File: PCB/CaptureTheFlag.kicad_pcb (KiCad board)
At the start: 2 copper layers, 96.5 x 61 mm, 11 parts, among them J1 Conn_01x04, J2 Conn_01x04, J3 Conn_01x08, J4 Conn_01x02

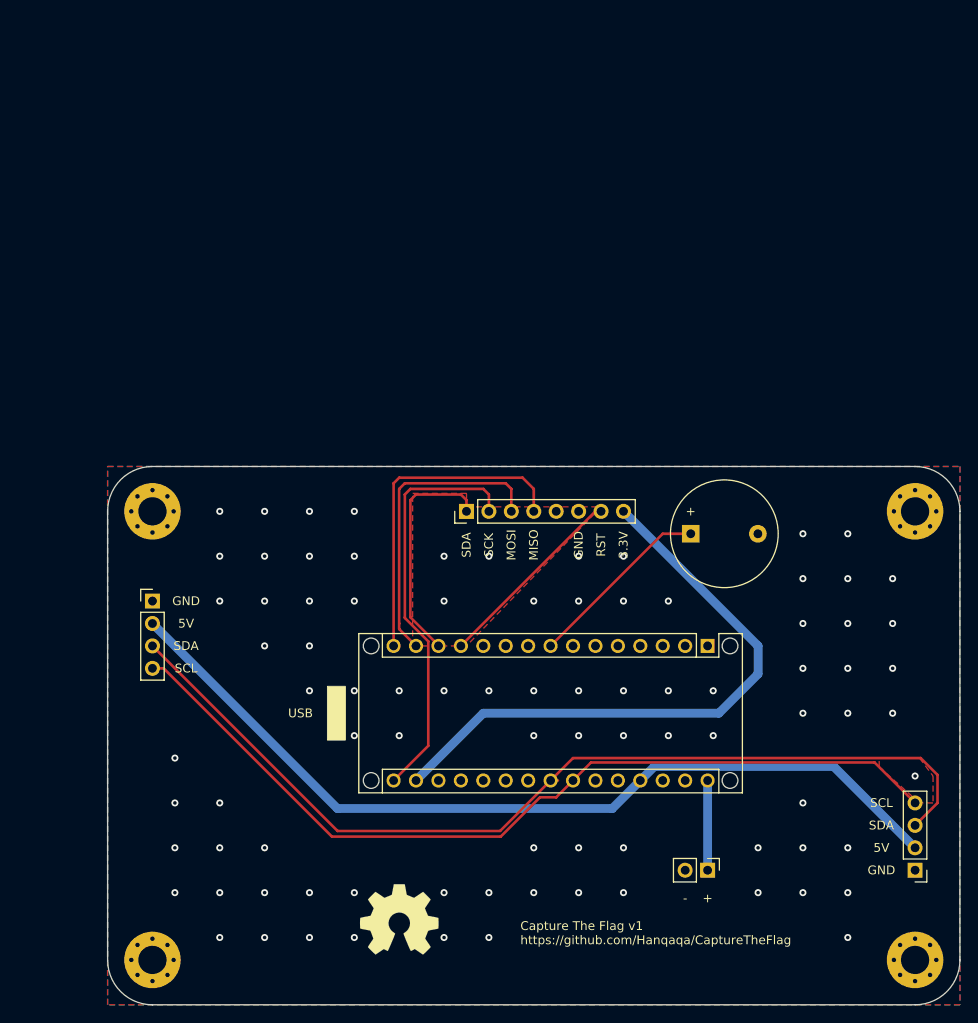
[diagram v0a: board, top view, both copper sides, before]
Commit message: v1.5
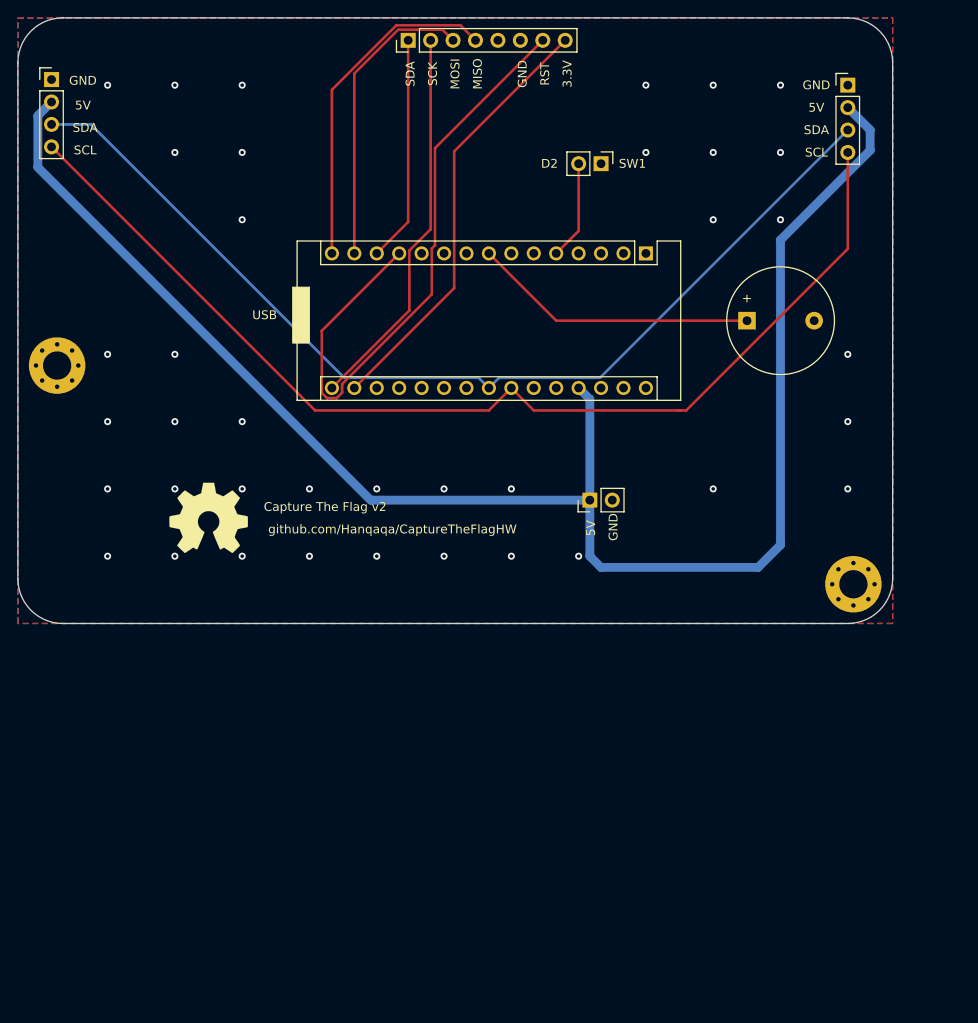
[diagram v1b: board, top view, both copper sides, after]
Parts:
- removed H3, H4: MountingHole_Pad, MountingHole:MountingHole_3.2mm_M3_Pad_Via
- added SW1: SW_DIP_x01, Connector_PinHeader_2.54mm:PinHeader_1x02_P2.54mm_Vertical, F.Cu at (170.2, 49.5)
- A1: footprint Module:Arduino_Nano_WithMountingHoles -> Module:Arduino_Nano
- moved H1 98.5 mm to (108.6, 72.4)
- moved J1 89.2 mm to (198.1, 40.6), turned to 0 degrees
- moved J2 60.2 mm to (108.0, 40.0)
- moved J3 53.7 mm to (148.3, 35.6)
- moved REF** 50.3 mm to (125.7, 89.7)
- moved A1 45.0 mm to (175.3, 59.7)
- moved J4 44.0 mm to (168.9, 87.6), turned to 90 degrees
- moved H2 43.1 mm to (198.8, 97.2)
- moved BZ1 25.0 mm to (186.7, 67.3)
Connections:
- J4 pad 1: VIN -> 5V
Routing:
- net 5V: track 100.8 -> 183.7 mm
- net SPI_RST: track 22.8 -> 71.6 mm
- net I2C_SCL: track 100.3 -> 123.5 mm
- net 3.3V: track 68.5 -> 49.3 mm
- net Net-(A1-Pad8): track 21.1 -> 32.4 mm
- net Net-(A1-Pad5): track 0.00 -> 11.2 mm
- net VIN: track 10.2 -> 0.00 mm
- net I2C_SDA: track 109.4 -> 114.6 mm
- net SPI_SCK: track 47.1 -> 44.0 mm
- net GND: vias 88 -> 38
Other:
- board size 96.5 x 61 mm -> 99.1 x 68.6 mm
- board text added: "Capture The Flag v2"
- board text added: "D2"
- board text added: "github.com/Hanqaqa/CaptureTheFlagHW"
- board text removed: "+"
- board text removed: "-"
- board text removed: "Capture The Flag v1 https://github.com/Hanqaqa/CaptureTheFlag"
